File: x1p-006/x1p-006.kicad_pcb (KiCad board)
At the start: 2 copper layers, 20.8 x 32.6 mm, 11 parts, among them U1 AD24C02, U3 TLP172GM(TPL,E(O, U6 TLP172GM(TPL,E(O

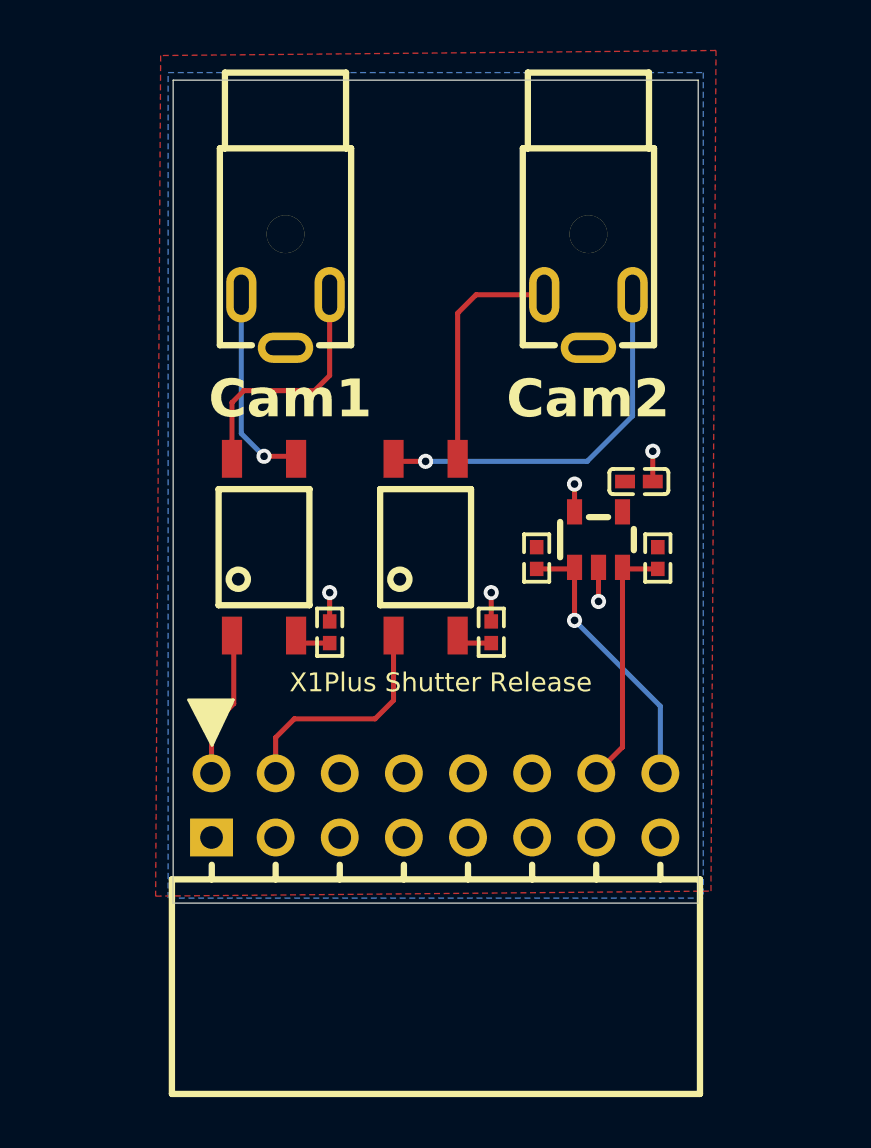
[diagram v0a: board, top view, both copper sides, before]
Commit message: x1p-006-b01
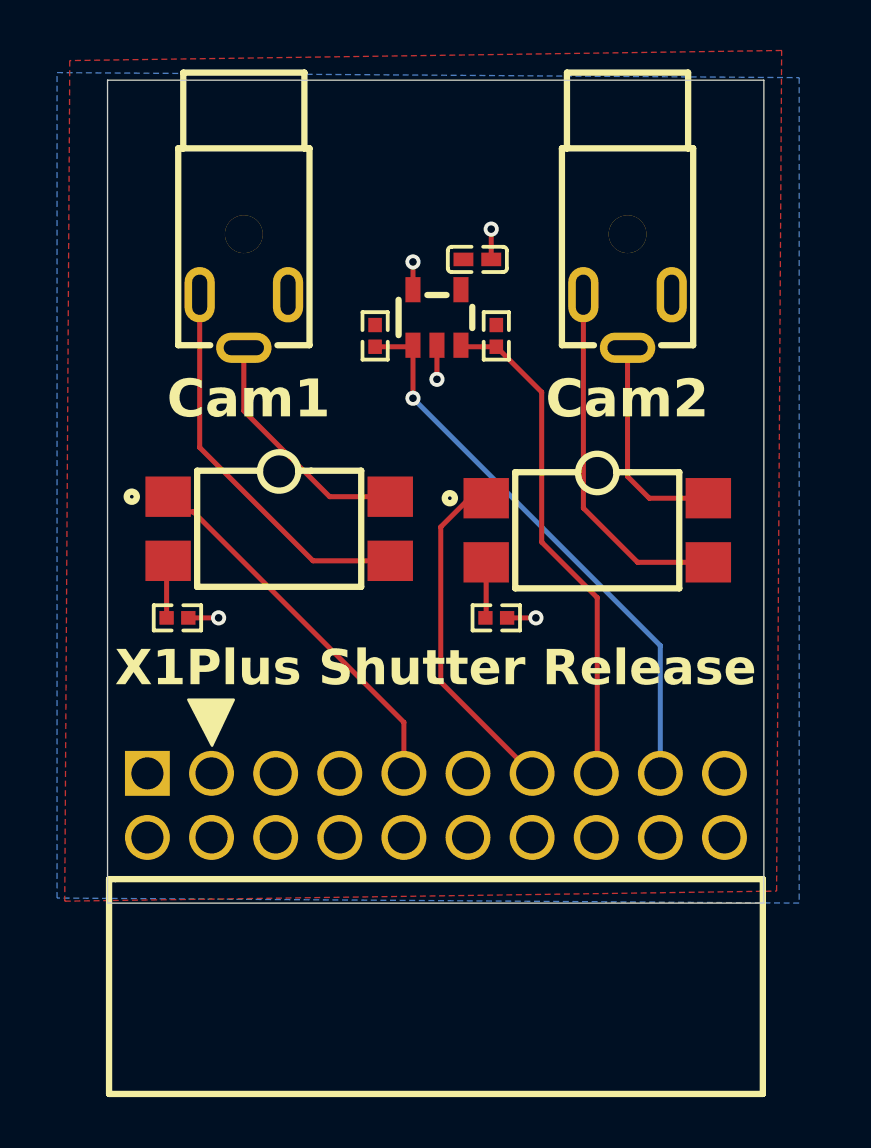
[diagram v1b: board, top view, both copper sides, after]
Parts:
- removed U6: TLP172GM(TPL,E(O, x1p-006:SMD-4_L4.6-W3.7-P2.54-LS7.0-BR
- added U2: TLP240A(TP1,F, x1p-006:RELAY-SMD_TLP240A, F.Cu at (62.2, 111.7)
- HDR1: value PM254-2-08-W-8.5 -> 220R-2*10P H=8.5MM Ytype Gold-plated black; footprint x1p-006:HDR-TH_16P-P2.54-H-F-R2-C8-W8.5 -> x1p-006:HDR-TH_20P-P2.54-H-F-R2-C10-S2.54-W10.2
- U3: value TLP172GM(TPL,E(O -> TLP240A(TP1,F; footprint x1p-006:SMD-4_L4.6-W3.7-P2.54-LS7.0-BR -> x1p-006:RELAY-SMD_TLP240A
- moved U3 13.2 mm to (74.8, 111.7)
- moved C1 10.9 mm to (70.0, 101.0)
- moved R1 10.9 mm to (66.0, 104.0)
- moved R2 10.9 mm to (70.8, 104.0)
- moved U1 10.9 mm to (68.5, 103.3)
- moved R3 6.06 mm to (58.2, 115.2), turned to 180 degrees
- moved PJ1 1.65 mm to (60.8, 103.5)
- moved PJ2 1.55 mm to (76.0, 103.5)
- moved R4 0.60 mm to (70.8, 115.2), turned to 180 degrees
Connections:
- HDR1 pad 1: GND -> unconnected-(HDR1-Pad1)
- HDR1 pad 11: 3V3 -> unconnected-(HDR1-Pad11)
- HDR1 pad 13: GND -> LD5
- HDR1 pad 14: LD6 -> 3V3
- HDR1 pad 15: GND -> LD6
- HDR1 pad 16: LD7 -> GND
- HDR1 pad 2: LD0 -> unconnected-(HDR1-Pad2)
- HDR1 pad 3: GND -> unconnected-(HDR1-Pad3)
- HDR1 pad 4: LD1 -> GND
- HDR1 pad 5: 3V3 -> unconnected-(HDR1-Pad5)
- HDR1 pad 6: unconnected-(HDR1-Pad6) -> GND
- HDR1 pad 8: unconnected-(HDR1-Pad8) -> 3V3
- HDR1 pad 9: unconnected-(HDR1-Pad9) -> LD3
- PJ1 pad 2: unconnected-(PJ1-Pad2) -> Net-(PJ1-Pad2)
- PJ1 pad 3: Net-(PJ1-Pad3) -> unconnected-(PJ1-Pad3)
- PJ2 pad 2: unconnected-(PJ2-Pad2) -> Net-(PJ2-Pad2)
- PJ2 pad 3: Net-(PJ2-Pad3) -> unconnected-(PJ2-Pad3)
- R3 pad 2: Net-(R3-Pad2) -> Net-(U2-C)
- R4 pad 2: Net-(R4-Pad2) -> Net-(U3-C)
- U3 pad 1: LD0 -> LD5
- U3 pad 2: Net-(R3-Pad2) -> Net-(U3-C)
- U3 pad 3: Net-(PJ1-Pad1) -> Net-(PJ2-Pad1)
- U3 pad 4: Net-(PJ1-Pad3) -> Net-(PJ2-Pad2)
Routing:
- net Net-(PJ2-Pad3): track 15.1 -> 0.00 mm, vias 1 -> 0
- net LD3: track 0.00 -> 14.8 mm
- net LD5: track 0.00 -> 13.5 mm
- net LD7: track 11.1 -> 22.5 mm
- net LD6: track 10.0 -> 20.0 mm
- net Net-(PJ1-Pad3): track 9.74 -> 0.00 mm
- net Net-(PJ1-Pad2): track 0.00 -> 9.71 mm
- net LD1: track 9.27 -> 0.00 mm
- net Net-(PJ2-Pad2): track 0.00 -> 8.66 mm
- net Net-(PJ1-Pad1): track 8.08 -> 15.5 mm, vias 1 -> 0
- net LD0: track 5.85 -> 0.00 mm
- net Net-(PJ2-Pad1): track 9.50 -> 14.3 mm
- net Net-(U2-C): track 0.00 -> 2.28 mm
- net Net-(U3-C): track 0.00 -> 2.20 mm
- net Net-(R3-Pad2): track 1.45 -> 0.00 mm
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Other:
- board size 20.8 x 32.6 mm -> 26 x 32.6 mm
- board text added: "X1P-006-B01"
- board text removed: "X1P-006-A01"
